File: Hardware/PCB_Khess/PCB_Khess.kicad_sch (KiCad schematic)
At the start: 13 parts, among them J1 Screw_Terminal_01x02, J2 Conn_01x02, J3 RJ11_Connector, J4 USB3_A, Q1 BUK9637-100E,118, U1 R-78B5.0-2.0

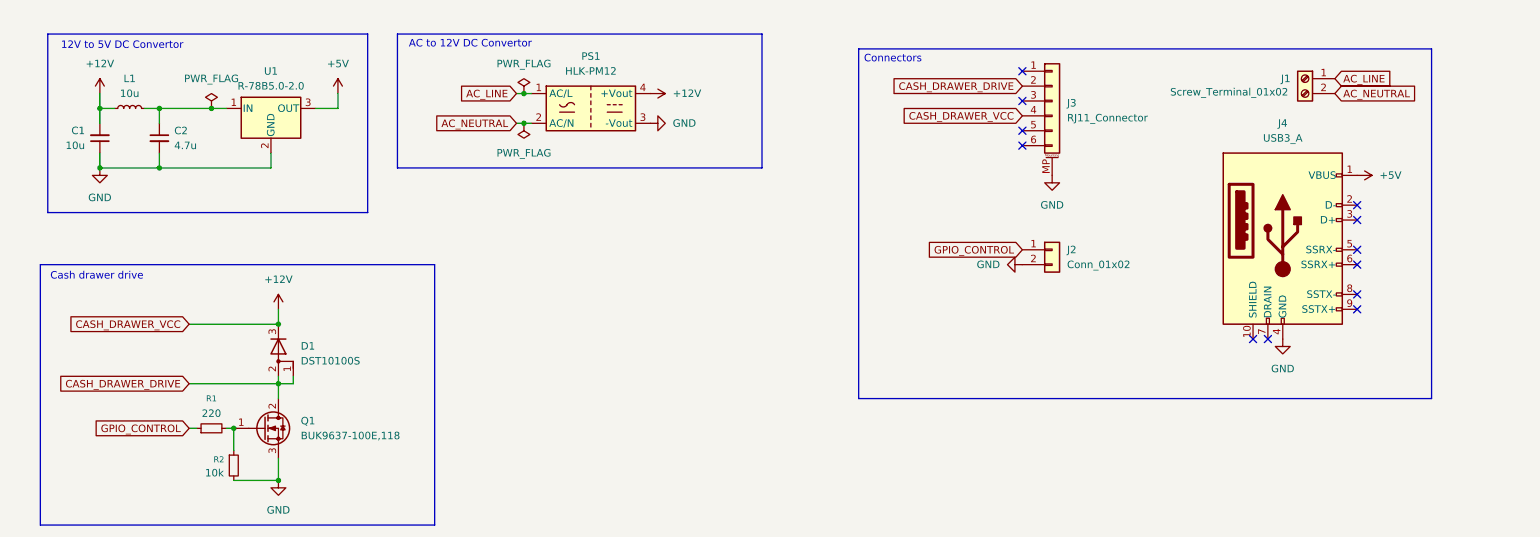
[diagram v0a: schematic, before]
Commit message: fix: update pcb
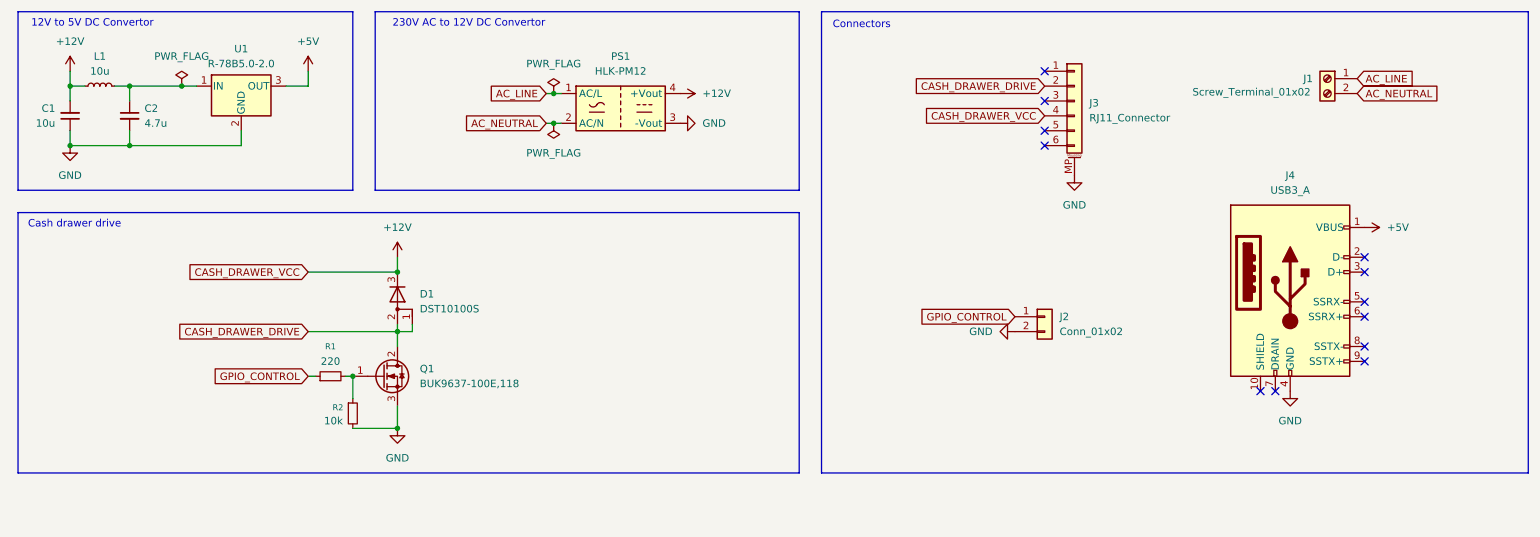
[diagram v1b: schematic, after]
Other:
- note added: "230V AC to 12V DC Convertor"
- note removed: "AC to 12V DC Convertor"
- moved on the sheet: C1, C2, D1, J1, J2, J3, J4, L1, PS1, Q1, R1, R2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
